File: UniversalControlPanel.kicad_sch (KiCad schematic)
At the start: 42 parts, among them J1 USB_B_Micro, J2 Conn_ARM_JTAG_SWD_10, J3 Conn_01x40, J4 Conn_02x03_Odd_Even, J5 Conn_01x02, J6 1Wire, J7 Conn_01x06, J8 Conn_01x07, J9 Conn_01x02, SW1 SW_Push, U1 TSR_1-2450, U2 MAX14783ExS, U3 USBLC6-2SC6, U4 AMS1117-3.3, U5 SN65HVD230, U6 ESP32-S2-WROOM-I

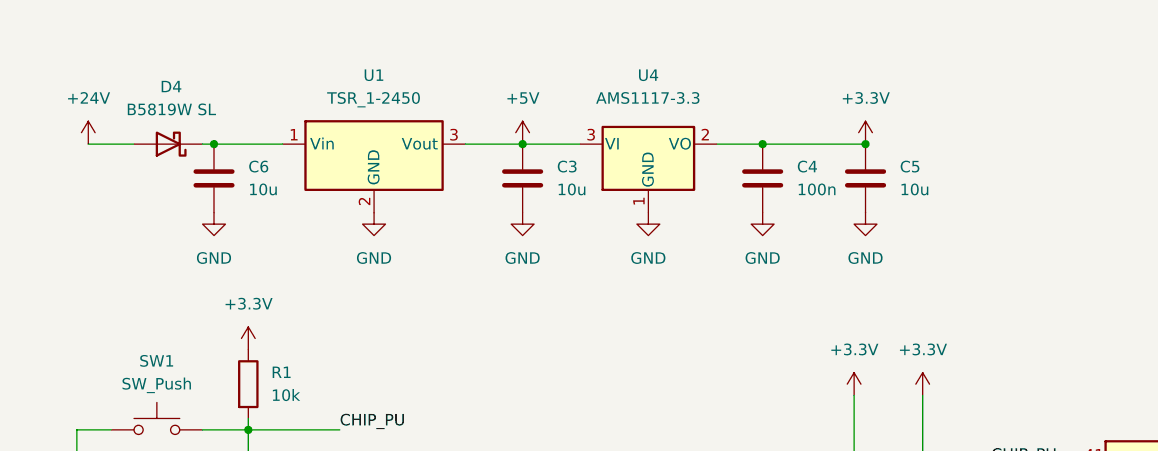
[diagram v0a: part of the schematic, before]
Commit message: placed
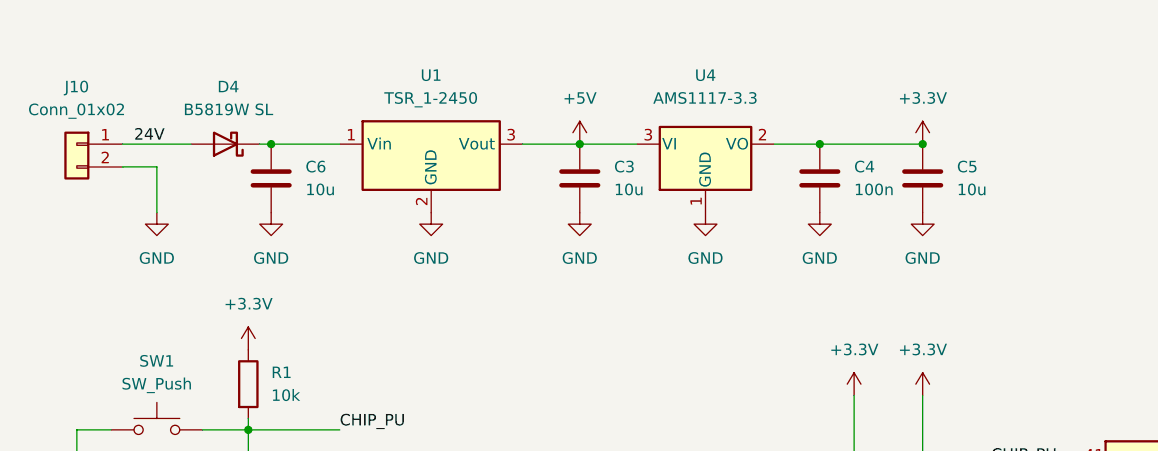
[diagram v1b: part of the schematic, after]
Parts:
- added J10: Conn_01x02, TerminalBlock_Phoenix:TerminalBlock_Phoenix_MKDS-1,5-2_1x02_P5.00mm_Horizontal, symbol Connector_Generic:Conn_01x02
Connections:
- net GND: now also J10.2 (Pin_2)
- net +24V renamed 24V
- net 24V: now also J10.1 (Pin_1)
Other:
- moved on the sheet: C3, C4, C5, C6, D4, U1, U4
